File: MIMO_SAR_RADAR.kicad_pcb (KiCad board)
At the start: 2 copper layers, 58 parts, among them IC1 SKY13418-485LF, IC10 ADL5380ACPZ-R7, IC11 AD7380-4BCPZ, IC2 SKY13418-485LF, IC3 SKY13418-485LF, IC4 LMX2594RHAT, IC5 LT3042IMSE#PBF, IC6 PSA2-6+, IC7 PSA2-6+, IC8 PMA3-73-1W+, IC9 ADL5380ACPZ-R7, J10 Conn_01x06_Pin, J3 SWD, J4 Conn_01x02_Pin, J5 Conn_Coaxial_Small, J6 Conn_Coaxial_Small, J7 Conn_01x06_Pin, J8 Conn_Coaxial_Small, J9 Conn_01x06_Pin, Q1 D44VH10, T1 TCM1-63AX-2+, T2 TCM1-63AX-2+, T3 TCM1-63AX-2+, T4 TCM1-63AX-2+, U1 STM32H745IITx, U2 ESP32-C3-WROOM-02, U3 LM2596S-12, U4 LM1117DT-3.3, U5 LM2596S-3.3, Y1 SiT9121AI-2B1-33E100.000000G

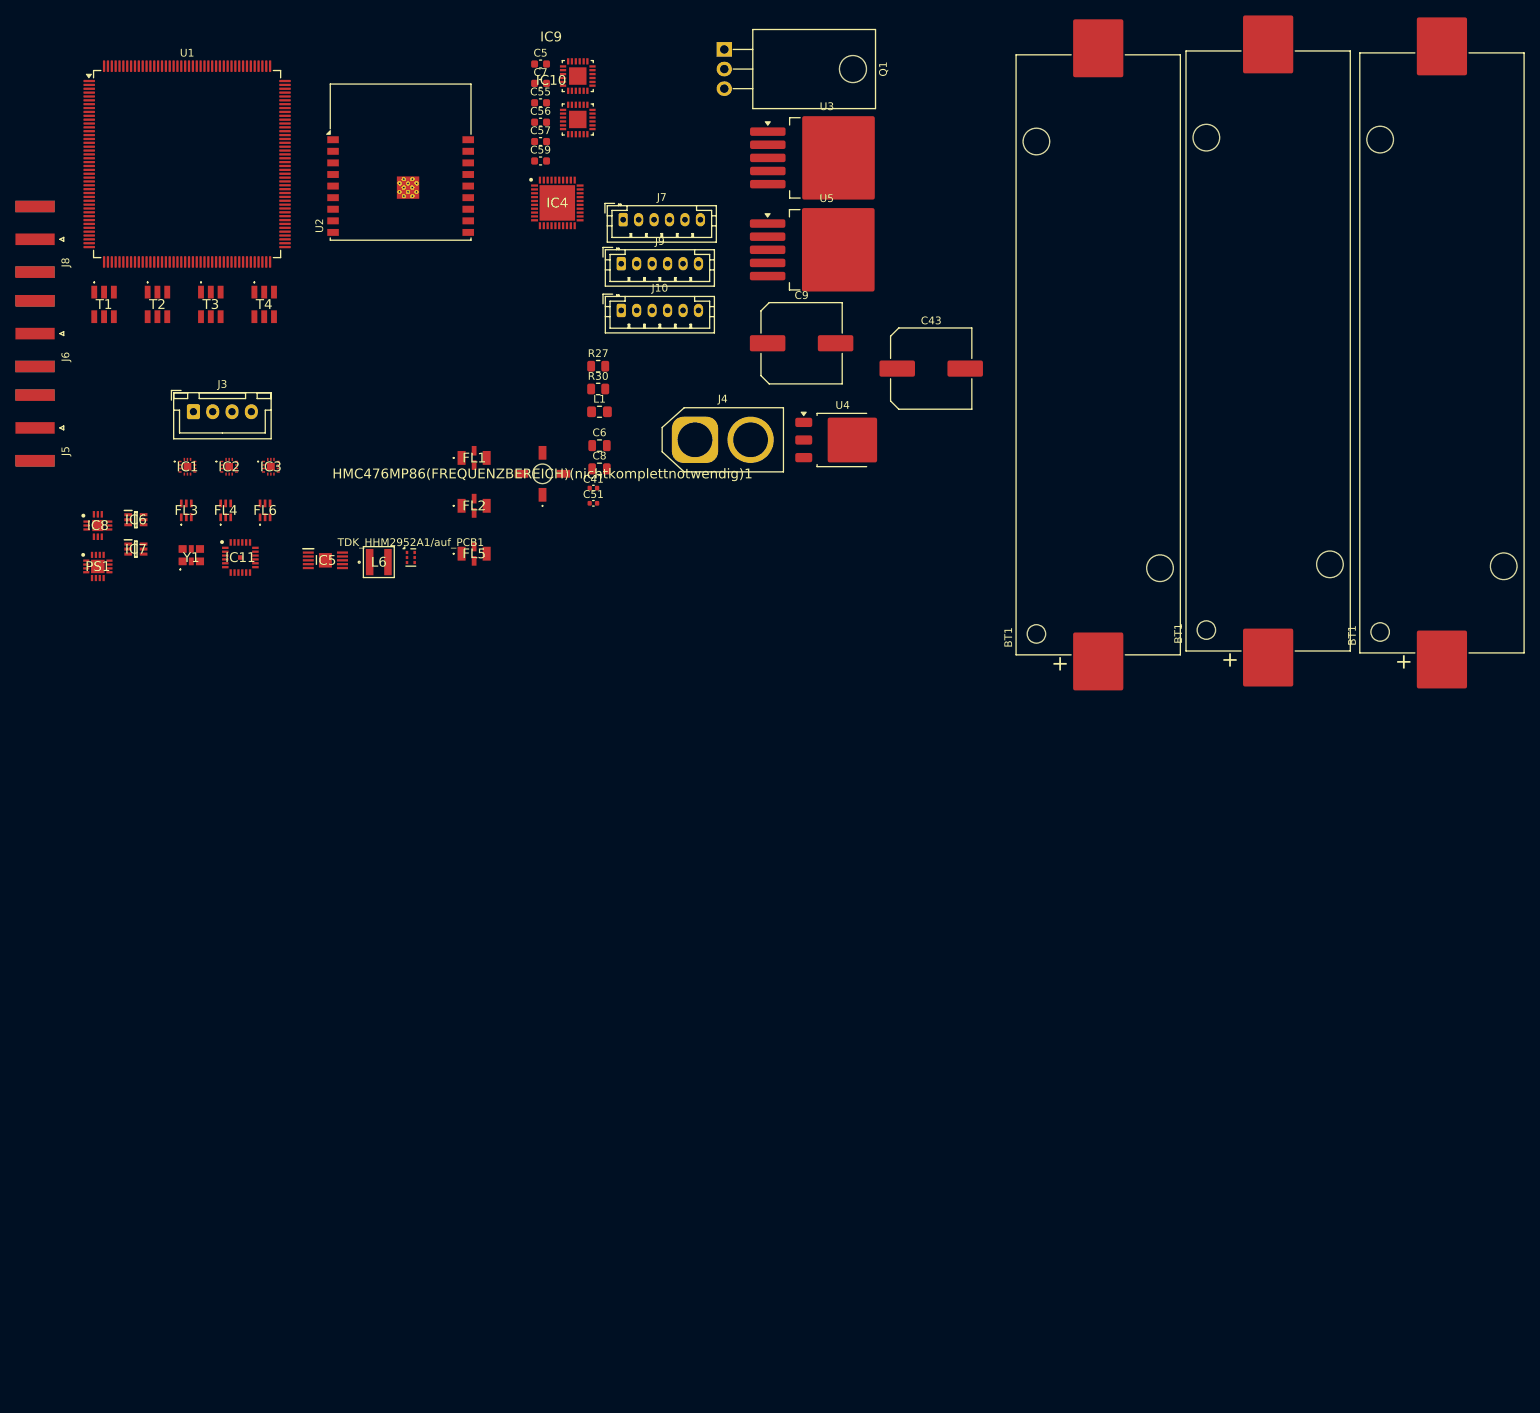
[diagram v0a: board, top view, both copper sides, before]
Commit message: layout
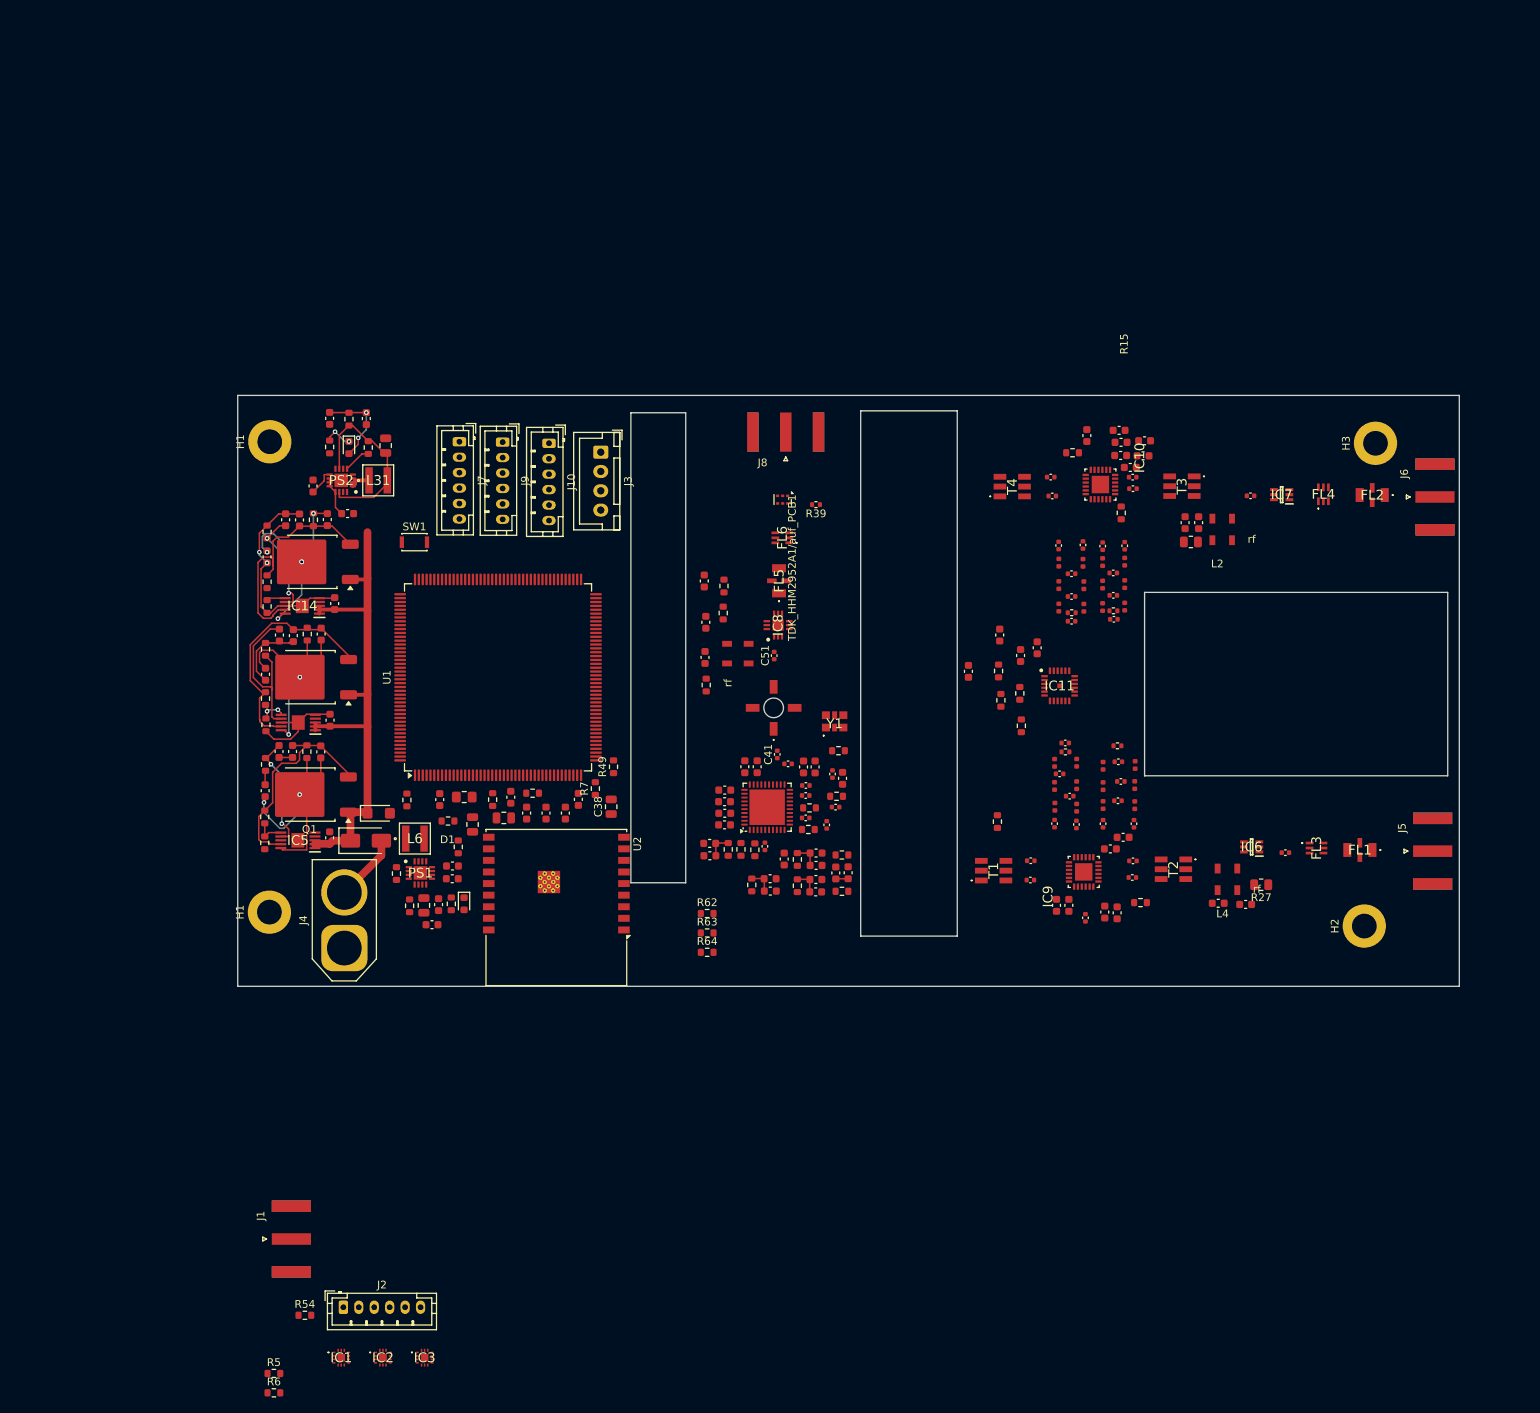
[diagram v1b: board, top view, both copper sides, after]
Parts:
- removed BT1 (x3): Battery_Cell, Battery:BatteryHolder_Keystone_1042_1x18650
- removed C43, C9: 680uF, Capacitor_SMD:C_Elec_10x10.2
- removed U3: LM2596S-12, Package_TO_SOT_SMD:TO-263-5_TabPin3
- removed U4: LM1117DT-3.3, Package_TO_SOT_SMD:TO-252-3_TabPin2
- removed U5: LM2596S-3.3, Package_TO_SOT_SMD:TO-263-5_TabPin3
- added C1: 2.2uF, Capacitor_SMD:C_0603_1608Metric, F.Cu at (94.0, 116.6)
- added C10: 0.1uF, Capacitor_SMD:C_0402_1005Metric, F.Cu at (134.0, 115.8)
- added C100: C_Small, Capacitor_SMD:C_0402_1005Metric, F.Cu at (163.7, 107.5)
- added C101: C_Small, Capacitor_SMD:C_0402_1005Metric, F.Cu at (170.6, 109.9)
- added C102: C_Small, Capacitor_SMD:C_0402_1005Metric, F.Cu at (164.6, 91.7)
- added C103: C_Small, Capacitor_SMD:C_0402_1005Metric, F.Cu at (170.0, 91.5)
- added C104: 1uF, Capacitor_SMD:C_0603_1608Metric, F.Cu at (160.1, 95.2)
- added C105: 1uF, Capacitor_SMD:C_0603_1608Metric, F.Cu at (151.2, 98.2)
- added C106: C_Small, Capacitor_SMD:C_0603_1608Metric, F.Cu at (155.2, 93.5)
- added C107: 1uF, Capacitor_SMD:C_0603_1608Metric, F.Cu at (157.9, 96.2)
- added C108: 10uF, Capacitor_SMD:C_0603_1608Metric, F.Cu at (70.8, 77.8)
- added C109: 4.7uF, Capacitor_SMD:C_0603_1608Metric, F.Cu at (68.5, 104.5)
- added C11: 0.1uF, Capacitor_SMD:C_0402_1005Metric, F.Cu at (133.6, 111.5)
- added C110: C_Small, Capacitor_SMD:C_0603_1608Metric, F.Cu at (60.2, 98.6)
- added C111: 10uF, Capacitor_SMD:C_0603_1608Metric, F.Cu at (67.4, 93.4)
- added C112: 0.47pF, Capacitor_SMD:C_0603_1608Metric, F.Cu at (62.0, 93.5)
- added C113: 10uF, Capacitor_SMD:C_0603_1608Metric, F.Cu at (63.8, 93.6)
- added C114: 3.3nF, Capacitor_SMD:C_0603_1608Metric, F.Cu at (66.3, 74.2)
- added C115: 22uF, Capacitor_SMD:C_0805_2012Metric, F.Cu at (75.8, 69.0)
- added C116: 0.1uF, Capacitor_SMD:C_0603_1608Metric, F.Cu at (68.5, 65.5)
- added C117: 10uF, Capacitor_SMD:C_0603_1608Metric, F.Cu at (73.2, 65.5)
- added C119: 4.7uF, Capacitor_SMD:C_0603_1608Metric, F.Cu at (69.2, 89.5)
- added C12: 0.1uF, Capacitor_SMD:C_0603_1608Metric, F.Cu at (131.3, 110.6)
- added C120: C_Small, Capacitor_SMD:C_0603_1608Metric, F.Cu at (60.4, 83.4)
- added C121: 10uF, Capacitor_SMD:C_0603_1608Metric, F.Cu at (68.2, 78.6)
- added C122: 0.47pF, Capacitor_SMD:C_0603_1608Metric, F.Cu at (62.8, 78.6)
- added C123: 10uF, Capacitor_SMD:C_0603_1608Metric, F.Cu at (64.6, 78.6)
- added C13: 0.1uF, Capacitor_SMD:C_0603_1608Metric, F.Cu at (134.0, 124.3)
- added C14: 0.1uF, Capacitor_SMD:C_0603_1608Metric, F.Cu at (131.4, 126.8)
- added C15: 0.1uF, Capacitor_SMD:C_0603_1608Metric, F.Cu at (131.5, 123.3)
- added C16: 0.1uF, Capacitor_SMD:C_0603_1608Metric, F.Cu at (117.7, 122.1)
- added C17: 0.1uF, Capacitor_SMD:C_0603_1608Metric, F.Cu at (125.5, 126.7)
- added C18: 10uF, Capacitor_SMD:C_0603_1608Metric, F.Cu at (129.8, 110.6)
- added C19: 1uF, Capacitor_SMD:C_0603_1608Metric, F.Cu at (135.6, 124.3)
- added C2: 100nF, Capacitor_SMD:C_0603_1608Metric, F.Cu at (96.5, 116.6)
- added C20: 1uF, Capacitor_SMD:C_0603_1608Metric, F.Cu at (131.4, 125.2)
- added C21: 10uF, Capacitor_SMD:C_0603_1608Metric, F.Cu at (131.5, 121.8)
- added C22: 1uF, Capacitor_SMD:C_0603_1608Metric, F.Cu at (117.7, 120.5)
- added C23: 10uF, Capacitor_SMD:C_0603_1608Metric, F.Cu at (125.5, 125.1)
- added C24: 10uF (X7R), Capacitor_SMD:C_0402_1005Metric, F.Cu at (124.8, 120.9)
- added C26: 1uF, Capacitor_SMD:C_0603_1608Metric, F.Cu at (127.3, 122.5)
- added C27: C_Small, Capacitor_SMD:C_0402_1005Metric, F.Cu at (130.1, 117.2)
- added C28: C_Small, Capacitor_SMD:C_0402_1005Metric, F.Cu at (132.8, 118.1)
- added C29: 1uF, Capacitor_SMD:C_0603_1608Metric, F.Cu at (119.6, 118.1)
- added C3: 4.7uF, Capacitor_SMD:C_0603_1608Metric, F.Cu at (99.0, 116.6)
- added C30: 10uF, Capacitor_SMD:C_0603_1608Metric, F.Cu at (119.7, 116.6)
- added C31: 4.7uF, Capacitor_SMD:C_0603_1608Metric, F.Cu at (68.5, 119.8)
- added C32: C_Small, Capacitor_SMD:C_0603_1608Metric, F.Cu at (119.6, 115.1)
- added C33: 10pF Np0/C0G 0402, Capacitor_SMD:C_0402_1005Metric, F.Cu at (130.1, 114.3)
- added C34: 10pF Np0/C0G 0402, Capacitor_SMD:C_0402_1005Metric, F.Cu at (130.2, 113.0)
- added C35: 10uF, Capacitor_SMD:C_0603_1608Metric, F.Cu at (119.7, 113.6)
- added C36: 1uF, Capacitor_SMD:C_0603_1608Metric, F.Cu at (123.8, 110.6)
- added C37: 10uF, Capacitor_SMD:C_0603_1608Metric, F.Cu at (134.9, 112.1)
- added C38: 10uF, Capacitor_SMD:C_0805_2012Metric, F.Cu at (105.0, 115.8)
- added C39: 10pF Np0/C0G 0402, Capacitor_SMD:C_0402_1005Metric, F.Cu at (127.8, 110.2)
- added C4: C_Small, Capacitor_SMD:C_0603_1608Metric, F.Cu at (100.7, 114.8)
- added C40: 10uF, Capacitor_SMD:C_0603_1608Metric, F.Cu at (122.2, 110.6)
- added C42: C_Small, Capacitor_SMD:C_0603_1608Metric, F.Cu at (60.1, 113.7)
- added C44: 10uF, Capacitor_SMD:C_0603_1608Metric, F.Cu at (67.3, 108.7)
- added C45: 0.47pF, Capacitor_SMD:C_0603_1608Metric, F.Cu at (62.0, 108.6)
- added C46: 2.2uF, Capacitor_SMD:C_0603_1608Metric, F.Cu at (117.1, 96.4)
- added C47: 2400pF, Capacitor_SMD:C_0402_1005Metric, F.Cu at (192.2, 121.7)
- added C48: 2400pF, Capacitor_SMD:C_0603_1608Metric, F.Cu at (174.0, 68.4)
- added C49: 1000pF, Capacitor_SMD:C_0603_1608Metric, F.Cu at (117.2, 91.9)
- added C50: 10uF, Capacitor_SMD:C_0603_1608Metric, F.Cu at (63.7, 108.6)
- added C52: 10uF, Capacitor_SMD:C_0603_1608Metric, F.Cu at (84.4, 123.4)
- added C53: 100pF, Capacitor_SMD:C_0603_1608Metric, F.Cu at (117.0, 86.5)
- added C54: 3.3nF, Capacitor_SMD:C_0603_1608Metric, F.Cu at (84.4, 125.1)
- added C58: 2400pF, Capacitor_SMD:C_0402_1005Metric, F.Cu at (166.3, 130.1)
- added C60: 2400pF, Capacitor_SMD:C_0402_1005Metric, F.Cu at (187.7, 75.5)
- added C61: 100pF, Capacitor_SMD:C_0603_1608Metric, F.Cu at (170.4, 129.5)
- added C62: 0.1uF, Capacitor_SMD:C_0603_1608Metric, F.Cu at (168.8, 129.4)
- added C63: 100pF, Capacitor_SMD:C_0603_1608Metric, F.Cu at (171.0, 68.6)
- added C64: 0.1uF, Capacitor_SMD:C_0603_1608Metric, F.Cu at (170.9, 70.3)
- added C65: 100pF, Capacitor_SMD:C_0603_1608Metric, F.Cu at (162.6, 128.5)
- added C66: 0.1uF, Capacitor_SMD:C_0603_1608Metric, F.Cu at (164.2, 128.5)
- added C67: 22uF, Capacitor_SMD:C_0805_2012Metric, F.Cu at (80.7, 128.5)
- added C68: 100pF, Capacitor_SMD:C_0603_1608Metric, F.Cu at (173.8, 70.3)
- added C69: 0.1uF, Capacitor_SMD:C_0603_1608Metric, F.Cu at (172.2, 71.8)
- added C70: 100pF, Capacitor_SMD:C_0402_1005Metric, F.Cu at (159.2, 125.2)
- added C71: 100pF, Capacitor_SMD:C_0402_1005Metric, F.Cu at (159.3, 122.7)
- added C72: 100pF, Capacitor_SMD:C_0402_1005Metric, F.Cu at (172.5, 122.8)
- added C73: 100pF, Capacitor_SMD:C_0402_1005Metric, F.Cu at (172.4, 124.9)
- added C74: 100pF, Capacitor_SMD:C_0402_1005Metric, F.Cu at (172.5, 73.1)
- added C75: 100pF, Capacitor_SMD:C_0402_1005Metric, F.Cu at (172.5, 74.6)
- added C76: 0.1uF, Capacitor_SMD:C_0603_1608Metric, F.Cu at (81.8, 131.0)
- added C77: 100pF, Capacitor_SMD:C_0402_1005Metric, F.Cu at (162.1, 75.5)
- added C78: 100pF, Capacitor_SMD:C_0402_1005Metric, F.Cu at (161.8, 73.1)
- added C79: 0.1uF, Capacitor_SMD:C_0603_1608Metric, F.Cu at (171.2, 119.7)
- added C80: 10uF, Capacitor_SMD:C_0603_1608Metric, F.Cu at (82.6, 128.4)
- added C81: 100pF, Capacitor_SMD:C_0603_1608Metric, F.Cu at (169.6, 121.2)
- added C82: 0.1uF, Capacitor_SMD:C_0603_1608Metric, F.Cu at (170.7, 67.0)
- added C83: 100pF, Capacitor_SMD:C_0603_1608Metric, F.Cu at (166.5, 67.7)
- added C84: 10uF, Capacitor_SMD:C_0402_1005Metric, F.Cu at (162.3, 117.9)
- added C85: 10uF, Capacitor_SMD:C_0402_1005Metric, F.Cu at (165.2, 118.0)
- added C86: 10uF, Capacitor_SMD:C_0402_1005Metric, F.Cu at (168.6, 118.0)
- added C87: 10uF, Capacitor_SMD:C_0402_1005Metric, F.Cu at (172.6, 118.0)
- added C88: 10uF, Capacitor_SMD:C_0402_1005Metric, F.Cu at (166.0, 81.9)
- added C89: 10uF, Capacitor_SMD:C_0402_1005Metric, F.Cu at (162.9, 81.9)
- added C90: 10uF, Capacitor_SMD:C_0402_1005Metric, F.Cu at (171.4, 82.0)
- added C91: 10uF, Capacitor_SMD:C_0402_1005Metric, F.Cu at (168.6, 82.0)
- added C92: C_Small, Capacitor_SMD:C_0402_1005Metric, F.Cu at (164.3, 114.4)
- added C93: C_Small, Capacitor_SMD:C_0402_1005Metric, F.Cu at (170.6, 115.0)
- added C94: C_Small, Capacitor_SMD:C_0402_1005Metric, F.Cu at (164.6, 85.6)
- added C95: C_Small, Capacitor_SMD:C_0402_1005Metric, F.Cu at (169.9, 85.5)
- added C96: C_Small, Capacitor_SMD:C_0402_1005Metric, F.Cu at (163.0, 111.5)
- added C97: C_Small, Capacitor_SMD:C_0402_1005Metric, F.Cu at (170.9, 112.5)
- added C98: C_Small, Capacitor_SMD:C_0402_1005Metric, F.Cu at (164.6, 88.5)
- added C99: C_Small, Capacitor_SMD:C_0402_1005Metric, F.Cu at (170.0, 88.4)
- added D1: SMF18A, Diode_SMD:D_SMF, F.Cu at (74.8, 116.6)
- added D3: VCO_POWER_CHECK, LED_SMD:LED_0603_1608Metric, F.Cu at (85.9, 128.3)
- added D4: VCO_POWER_CHECK, LED_SMD:LED_0603_1608Metric, F.Cu at (71.0, 69.2)
- added D5: SS54, Diode_SMD:D_SMA, F.Cu at (73.2, 120.2)
- added H1: MountingHole, MountingHole:MountingHole_3.2mm_M3_DIN965_Pad, F.Cu at (60.7, 129.4)
- added H1: MountingHole, MountingHole:MountingHole_3.2mm_M3_DIN965_Pad, F.Cu at (60.8, 68.5)
- added H2: MountingHole, MountingHole:MountingHole_3.2mm_M3_DIN965_Pad, F.Cu at (202.4, 131.2)
- added H3: MountingHole, MountingHole:MountingHole_3.2mm_M3_DIN965_Pad, F.Cu at (203.9, 68.7)
- added IC12: LT3042IMSE#PBF, Low_noise_LDO:SOP50P490X110-11N, F.Cu at (64.4, 104.8)
- added IC14: LT3042IMSE#PBF, Low_noise_LDO:SOP50P490X110-11N, F.Cu at (65.0, 89.8)
- added J1: Conn_Coaxial_Small, Connector_Coaxial:SMA_Amphenol_132289_EdgeMount, F.Cu at (63.5, 171.7)
- added J2: Conn_01x06_Pin, Connector_JST:JST_PH_B6B-PH-K_1x06_P2.00mm_Vertical, F.Cu at (70.3, 180.5)
- added L10: L_Small, Inductor_SMD:L_0402_1005Metric, F.Cu at (172.7, 115.5)
- added L11: L_Small, Inductor_SMD:L_0402_1005Metric, F.Cu at (166.0, 84.2)
- added L12: L_Small, Inductor_SMD:L_0402_1005Metric, F.Cu at (162.9, 84.1)
- added L13: L_Small, Inductor_SMD:L_0402_1005Metric, F.Cu at (171.4, 84.0)
- added L14: L_Small, Inductor_SMD:L_0402_1005Metric, F.Cu at (168.6, 84.1)
- added L15: L_Small, Inductor_SMD:L_0402_1005Metric, F.Cu at (162.3, 113.1)
- added L16: L_Small, Inductor_SMD:L_0402_1005Metric, F.Cu at (165.2, 113.0)
- added L17: L_Small, Inductor_SMD:L_0402_1005Metric, F.Cu at (168.6, 113.1)
- added L18: L_Small, Inductor_SMD:L_0402_1005Metric, F.Cu at (172.7, 112.9)
- added L19: L_Small, Inductor_SMD:L_0402_1005Metric, F.Cu at (166.1, 87.1)
- added L2: TCCH-80, TCCH-80:GU1604, F.Cu at (184.1, 79.8)
- added L20: L_Small, Inductor_SMD:L_0402_1005Metric, F.Cu at (162.9, 87.1)
- added L21: L_Small, Inductor_SMD:L_0402_1005Metric, F.Cu at (171.4, 86.9)
- added L22: L_Small, Inductor_SMD:L_0402_1005Metric, F.Cu at (168.6, 87.0)
- added L23: L_Small, Inductor_SMD:L_0402_1005Metric, F.Cu at (162.3, 110.1)
- added L24: L_Small, Inductor_SMD:L_0402_1005Metric, F.Cu at (165.2, 110.0)
- added L25: L_Small, Inductor_SMD:L_0402_1005Metric, F.Cu at (168.6, 110.4)
- added L26: L_Small, Inductor_SMD:L_0402_1005Metric, F.Cu at (172.8, 110.3)
- added L27: L_Small, Inductor_SMD:L_0402_1005Metric, F.Cu at (166.1, 90.0)
- added L28: L_Small, Inductor_SMD:L_0402_1005Metric, F.Cu at (162.9, 90.0)
- added L29: L_Small, Inductor_SMD:L_0402_1005Metric, F.Cu at (171.4, 89.8)
- added L30: L_Small, Inductor_SMD:L_0402_1005Metric, F.Cu at (168.6, 89.9)
- added L31: XFL4020-222MEB, XFL4020-222:XFL4020-222ME, F.Cu at (74.8, 73.5)
- added L4: TCCH-80, TCCH-80:GU1604, F.Cu at (184.7, 125.2)
- added L5: TCCH-80, TCCH-80:GU1604, F.Cu at (121.3, 95.9)
- added L7: L_Small, Inductor_SMD:L_0402_1005Metric, F.Cu at (162.4, 115.7)
- added L8: L_Small, Inductor_SMD:L_0402_1005Metric, F.Cu at (165.2, 115.9)
- added L9: L_Small, Inductor_SMD:L_0402_1005Metric, F.Cu at (168.6, 115.5)
- added PS2: TPS62150RGTR, TPS62150:QFN50P300X300X100-17N-D, F.Cu at (70.0, 73.5)
- added Q2: DPAK, Package_TO_SOT_SMD:TO-252-2, F.Cu at (65.9, 99.0)
- added Q4: D44VH10, Package_TO_SOT_SMD:TO-252-2, F.Cu at (66.1, 84.0)
- added R1: 10k, Resistor_SMD:R_0603_1608Metric, F.Cu at (78.5, 114.9)
- added R10: 1.5R, Resistor_SMD:R_0603_1608Metric, F.Cu at (134.8, 126.7)
- added R11: 1.5R, Resistor_SMD:R_0603_1608Metric, F.Cu at (129.1, 126.0)
- added R12: 1.5R, Resistor_SMD:R_0603_1608Metric, F.Cu at (129.1, 122.6)
- added R13: 1.5R, Resistor_SMD:R_0603_1608Metric, F.Cu at (120.1, 121.3)
- added R14: 1.5R, Resistor_SMD:R_0603_1608Metric, F.Cu at (123.2, 125.9)
- added R15: 10k, Resistor_SMD:R_0603_1608Metric, F.Cu at (121.8, 121.3)
- added R16: R_Small, Resistor_SMD:R_0603_1608Metric, F.Cu at (123.5, 121.3)
- added R17: werte_siehe_PLLATINUM_SIM, Resistor_SMD:R_0603_1608Metric, F.Cu at (130.6, 115.9)
- added R19: R_Small, Resistor_SMD:R_0603_1608Metric, F.Cu at (134.8, 122.0)
- added R2: R_Small, Resistor_SMD:R_0603_1608Metric, F.Cu at (89.6, 114.8)
- added R20: R_Small, Resistor_SMD:R_0603_1608Metric, F.Cu at (130.5, 118.7)
- added R21: 10k, Resistor_SMD:R_0603_1608Metric, F.Cu at (65.5, 108.6)
- added R22: 50k, Resistor_SMD:R_0603_1608Metric, F.Cu at (60.2, 110.3)
- added R23: 240R, Resistor_SMD:R_0603_1608Metric, F.Cu at (117.2, 100.0)
- added R24: 249k, Resistor_SMD:R_0603_1608Metric, F.Cu at (60.1, 117.1)
- added R25: 49k, Resistor_SMD:R_0603_1608Metric, F.Cu at (60.1, 120.4)
- added R28: 180k, Resistor_SMD:R_0603_1608Metric, F.Cu at (77.2, 124.4)
- added R29: R_Small, Resistor_SMD:R_0603_1608Metric, F.Cu at (119.5, 90.7)
- added R3: inf, Resistor_SMD:R_0603_1608Metric, F.Cu at (83.8, 117.6)
- added R31: R_Small, Resistor_SMD:R_0603_1608Metric, F.Cu at (119.5, 87.2)
- added R32: 562k, Resistor_SMD:R_0603_1608Metric, F.Cu at (78.8, 128.6)
- added R33: 0R, Resistor_SMD:R_0603_1608Metric, F.Cu at (173.5, 128.2)
- added R34: 0R, Resistor_SMD:R_0603_1608Metric, F.Cu at (164.7, 69.9)
- added R35: 0R, Resistor_SMD:R_0603_1608Metric, F.Cu at (84.2, 128.3)
- added R36: 200R, Resistor_SMD:R_0603_1608Metric, F.Cu at (154.9, 117.7)
- added R37: 200R, Resistor_SMD:R_0603_1608Metric, F.Cu at (171.0, 77.7)
- added R38: R_Small, Resistor_SMD:R_0603_1608Metric, F.Cu at (85.2, 121.0)
- added R39: 0402 RF 50 Ohm thin film, Resistor_SMD:R_0402_1005Metric, F.Cu at (131.5, 76.6)
- added R4: 10k, Resistor_SMD:R_0603_1608Metric, F.Cu at (94.8, 114.0)
- added R40: 500R, Resistor_SMD:R_0402_1005Metric, F.Cu at (163.8, 108.7)
- added R41: 500R, Resistor_SMD:R_0402_1005Metric, F.Cu at (170.5, 107.9)
- added R42: 500R, Resistor_SMD:R_0402_1005Metric, F.Cu at (164.6, 90.6)
- added R43: 500R, Resistor_SMD:R_0402_1005Metric, F.Cu at (170.0, 90.4)
- added R44: R_Small, Resistor_SMD:R_0603_1608Metric, F.Cu at (157.8, 101.1)
- added R45: R_Small, Resistor_SMD:R_0603_1608Metric, F.Cu at (158.1, 105.3)
- added R46: R_Small, Resistor_SMD:R_0603_1608Metric, F.Cu at (155.4, 102.0)
- added R47: R_Small, Resistor_SMD:R_0603_1608Metric, F.Cu at (155.1, 98.2)
- added R49: R_Small, Resistor_SMD:R_0603_1608Metric, F.Cu at (105.2, 110.6)
- added R5: 0R, Resistor_SMD:R_0603_1608Metric, F.Cu at (61.3, 189.1)
- added R50: 10k, Resistor_SMD:R_0603_1608Metric, F.Cu at (65.6, 93.4)
- added R51: 121k, Resistor_SMD:R_0603_1608Metric, F.Cu at (60.2, 95.4)
- added R52: 249k, Resistor_SMD:R_0603_1608Metric, F.Cu at (60.2, 101.8)
- added R53: 49k, Resistor_SMD:R_0603_1608Metric, F.Cu at (60.2, 105.2)
- added R54: 180k, Resistor_SMD:R_0603_1608Metric, F.Cu at (65.3, 181.6)
- added R55: 562k, Resistor_SMD:R_0603_1608Metric, F.Cu at (73.5, 69.2)
- added R56: 0R, Resistor_SMD:R_0603_1608Metric, F.Cu at (71.0, 65.6)
- added R57: R_Small, Resistor_SMD:R_0603_1608Metric, F.Cu at (68.5, 69.2)
- added R58: 10k, Resistor_SMD:R_0603_1608Metric, F.Cu at (66.4, 78.6)
- added R59: 33k, Resistor_SMD:R_0603_1608Metric, F.Cu at (60.4, 80.2)
- added R6: 0R, Resistor_SMD:R_0603_1608Metric, F.Cu at (61.3, 191.6)
- added R60: 249k, Resistor_SMD:R_0603_1608Metric, F.Cu at (60.4, 86.6)
- added R61: 49k, Resistor_SMD:R_0603_1608Metric, F.Cu at (60.4, 89.8)
- added R62: 0R, Resistor_SMD:R_0603_1608Metric, F.Cu at (117.4, 129.6)
- added R63: 0R, Resistor_SMD:R_0603_1608Metric, F.Cu at (117.4, 132.1)
- added R64: 0R, Resistor_SMD:R_0603_1608Metric, F.Cu at (117.4, 134.6)
- added R7: R_Small, Resistor_SMD:R_0603_1608Metric, F.Cu at (102.9, 113.4)
- added R8: 100R, Resistor_SMD:R_0603_1608Metric, F.Cu at (134.1, 114.4)
- added R9: 1.5R, Resistor_SMD:R_0603_1608Metric, F.Cu at (134.4, 108.5)
- added SW1: SW_Push, Button_Switch_SMD:SW_SPST_CK_KXT3, F.Cu at (79.5, 81.5)
- IC4: footprint LMX:QFN50P600X600X100-41N-D -> Package_DFN_QFN:QFN-40-1EP_6x6mm_P0.5mm_EP4.6x4.6mm
- Q1: footprint Package_TO_SOT_THT:TO-220-3_Horizontal_TabDown -> Package_TO_SOT_SMD:TO-252-2
- moved J5 189.1 mm to (211.3, 121.5), turned to 0 degrees
- moved J6 182.5 mm to (211.6, 75.7), turned to 0 degrees
- moved FL3 152.7 mm to (196.3, 121.1), turned to -90 degrees
- moved IC6 150.5 mm to (187.9, 121.0), turned to 180 degrees
- moved T2 150.5 mm to (177.7, 123.8), turned to -90 degrees
- moved IC7 148.5 mm to (191.8, 75.3), turned to 180 degrees
- moved FL4 142.1 mm to (197.2, 75.3)
- moved C55 138.2 mm to (187.1, 128.4), turned to 180 degrees
- moved T1 136.5 mm to (154.5, 124.0), turned to 90 degrees
- moved C57 132.0 mm to (183.5, 128.2), turned to 180 degrees
- moved T3 127.9 mm to (178.8, 74.3), turned to -90 degrees
- moved FL1 125.4 mm to (201.9, 121.3), turned to 180 degrees
- moved IC9 122.1 mm to (166.1, 124.2), turned to 90 degrees
- moved IC1 117.0 mm to (70.0, 187.1)
- moved IC2 117.0 mm to (75.4, 187.1)
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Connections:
- IC11 pad 4: VDDSMPS -> VCC_ADC
- IC5 pad 1: +12V -> BAT+
- IC5 pad 2: +12V -> BAT+
- IC5 pad 3: +12V -> BAT+
- IC5 pad 9: 5V_CLEAN -> Net-(IC5-OUTS)
- PS1 pad 10: Net-(PS1-AVIN) -> BAT+
- PS1 pad 11: Net-(PS1-AVIN) -> BAT+
- PS1 pad 12: Net-(PS1-AVIN) -> BAT+
- PS1 pad 13: Net-(PS1-AVIN) -> BAT+
- Q1 pad 1: +12V -> BAT+
- Q1 pad 3: 5V_CLEAN -> Net-(IC5-OUTS)
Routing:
- net BAT+: track 0.00 -> 72.4 mm
- net VSS: track 0.00 -> 53.2 mm, vias 0 -> 2
- net Net-(IC5-OUT): track 0.00 -> 32.7 mm, vias 0 -> 2
- net Net-(IC12-OUT): track 0.00 -> 31.5 mm, vias 0 -> 2
- net Net-(IC12-OUTS): track 0.00 -> 30.7 mm
- net Net-(IC14-OUTS): track 0.00 -> 30.7 mm
- net Net-(IC5-OUTS): track 0.00 -> 28.2 mm
- net Net-(IC14-OUT): track 0.00 -> 27.8 mm, vias 0 -> 5
- net Net-(PS2-FSW): track 0.00 -> 24.0 mm
- net Net-(IC12-SET): track 0.00 -> 21.1 mm
- net Net-(IC5-SET): track 0.00 -> 14.9 mm, vias 0 -> 2
- net Net-(IC14-SET): track 0.00 -> 13.9 mm, vias 0 -> 2
- net VDDSMPS: track 0.00 -> 11.0 mm, vias 0 -> 2
- net Net-(D5-A): track 0.00 -> 8.69 mm
- net Net-(IC12-PGFB): track 0.00 -> 4.20 mm, vias 0 -> 2
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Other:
- board outline added: 158.2 x 76.5 mm
